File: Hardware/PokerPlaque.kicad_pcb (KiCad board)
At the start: 2 copper layers, 40 x 33 mm, 7 parts, among them J1 Conn_01x05_Pin, J2 Conn_01x04_Pin, J3 Conn_01x02_Pin, J4 Conn_01x08_Pin, U1 CH32V203C8T6

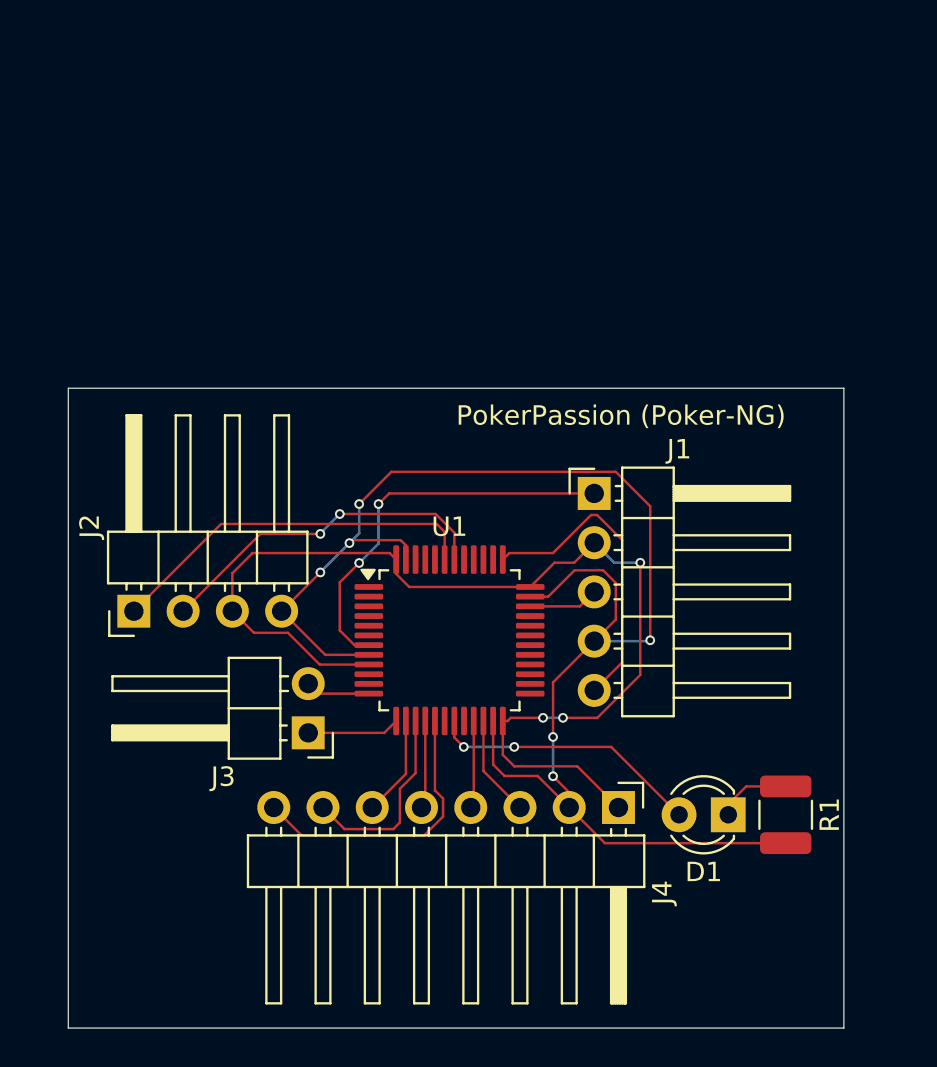
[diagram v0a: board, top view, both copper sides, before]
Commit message: feat: added some necessities
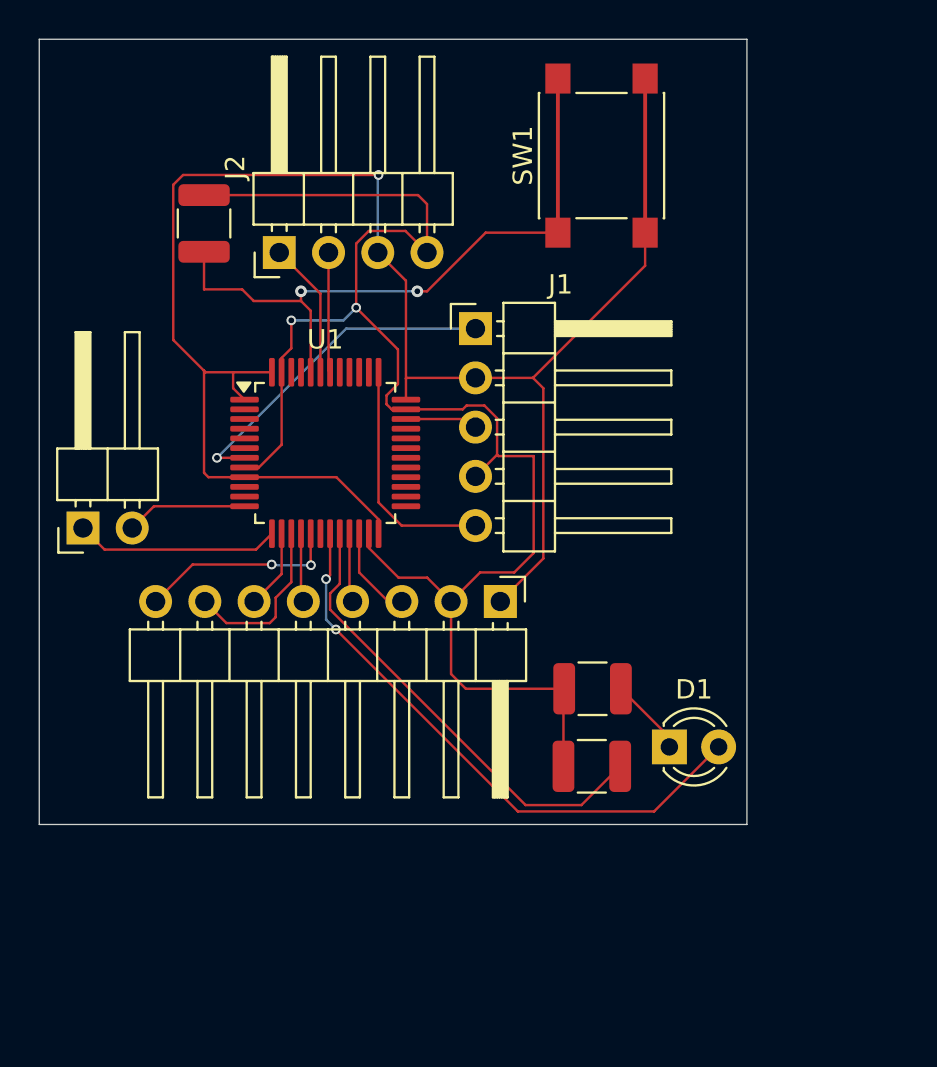
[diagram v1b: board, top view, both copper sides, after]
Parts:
- added R2: 10k Ohm, Resistor_SMD:R_1210_3225Metric, F.Cu at (30.5, 29.5)
- added R3: 10k Ohm, Resistor_SMD:R_1210_3225Metric, F.Cu at (50.5, 57.5)
- added SW1: KH-6X6X6H-STM, Button_Switch_SMD:SW_Push_1P1T_NO_6x6mm_H9.5mm, F.Cu at (51.0, 26.0)
- D1: value NFD3401URD LED -> NFD3401URD
- J1: value Conn_01x05_Pin -> A2541WR-5P
- J2: value Conn_01x04_Pin -> A2541WR-4P
- J3: value Conn_01x02_Pin -> A2541WR-2P
- J4: value Conn_01x08_Pin -> A2541WR-8P
- moved J2 20.0 mm to (34.4, 31.0)
- moved J3 15.7 mm to (24.3, 45.2), turned to 90 degrees
- moved J4 12.2 mm to (45.8, 49.0)
- moved R1 11.9 mm to (50.5, 53.5), turned to 180 degrees
- moved U1 11.6 mm to (36.8, 41.3)
- moved J1 10.5 mm to (44.5, 34.9)
- moved D1 4.64 mm to (54.5, 56.5), turned to 0 degrees
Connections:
- U1 pad 1: unconnected-(U1-VBAT-Pad1) -> +3.3V
- U1 pad 20: unconnected-(U1-PB2-Pad20) -> BOOT1
- U1 pad 44: unconnected-(U1-BOOT0-Pad44) -> BOOT0
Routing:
- net +3.3V: track 56.8 -> 91.5 mm, vias 3 -> 1
- net BOOT0: track 0.00 -> 34.0 mm, vias 0 -> 2
- net BOOT1: track 0.00 -> 24.1 mm
- net DEBUG_LED0: track 14.1 -> 30.2 mm
- net I2C1_SDA: track 19.5 -> 7.05 mm
- net I2C1_SCL: track 17.9 -> 6.21 mm, vias 2 -> 0
- net RESERVED_UART_RX: track 4.79 -> 10.5 mm
- net DISPLAY_MOSI1: track 14.8 -> 10.5 mm, vias 0 -> 2
- net SWCLK: track 16.0 -> 12.2 mm
- net RST: track 20.5 -> 17.5 mm, vias 2 -> 1
- net RESERVED_UART_TX: track 3.34 -> 6.26 mm
- net GND: track 80.2 -> 82.5 mm, vias 6 -> 2
- net DISPLAY_SCK1: track 10.1 -> 8.88 mm
- net DISPLAY_SS1: track 5.18 -> 4.09 mm
- net DISPLAY_MISO1: track 4.54 -> 3.55 mm
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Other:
- board size 40 x 33 mm -> 36.5 x 40.5 mm
- board text removed: "PokerPassion (Poker-NG)"
